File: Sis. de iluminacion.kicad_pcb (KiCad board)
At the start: 2 copper layers, 86.8 x 98.1 mm, 48 parts, among them J1 Screw_Terminal_01x02, J10 Screw_Terminal_01x02, J11 Screw_Terminal_01x02, J12 Screw_Terminal_01x02, J3 Screw_Terminal_01x02, J4 Conn_01x04, J5 Screw_Terminal_01x02, J7 Screw_Terminal_01x02, J8 Screw_Terminal_01x02, J9 Screw_Terminal_01x02, K10 Relay_DPDT, K11 Relay_DPDT, K8 Relay_DPDT, K9 Relay_DPDT, Q4 BC547, Q5 BC547, Q6 BC547, Q7 BC547, U1 ESP32_DEVKITC, U10 PC817, U11 PC817, U12 PC817, U13 PC817, U3 L7805

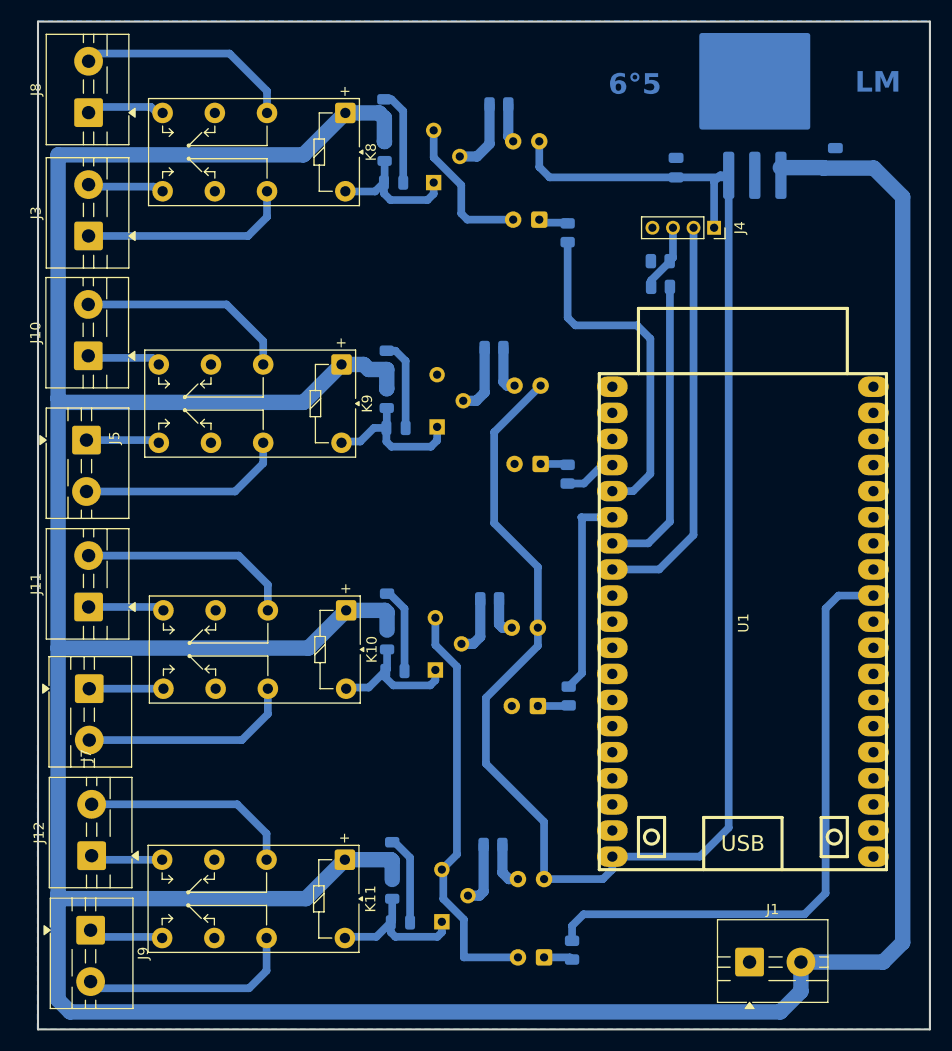
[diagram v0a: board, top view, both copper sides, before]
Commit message: Add files via upload
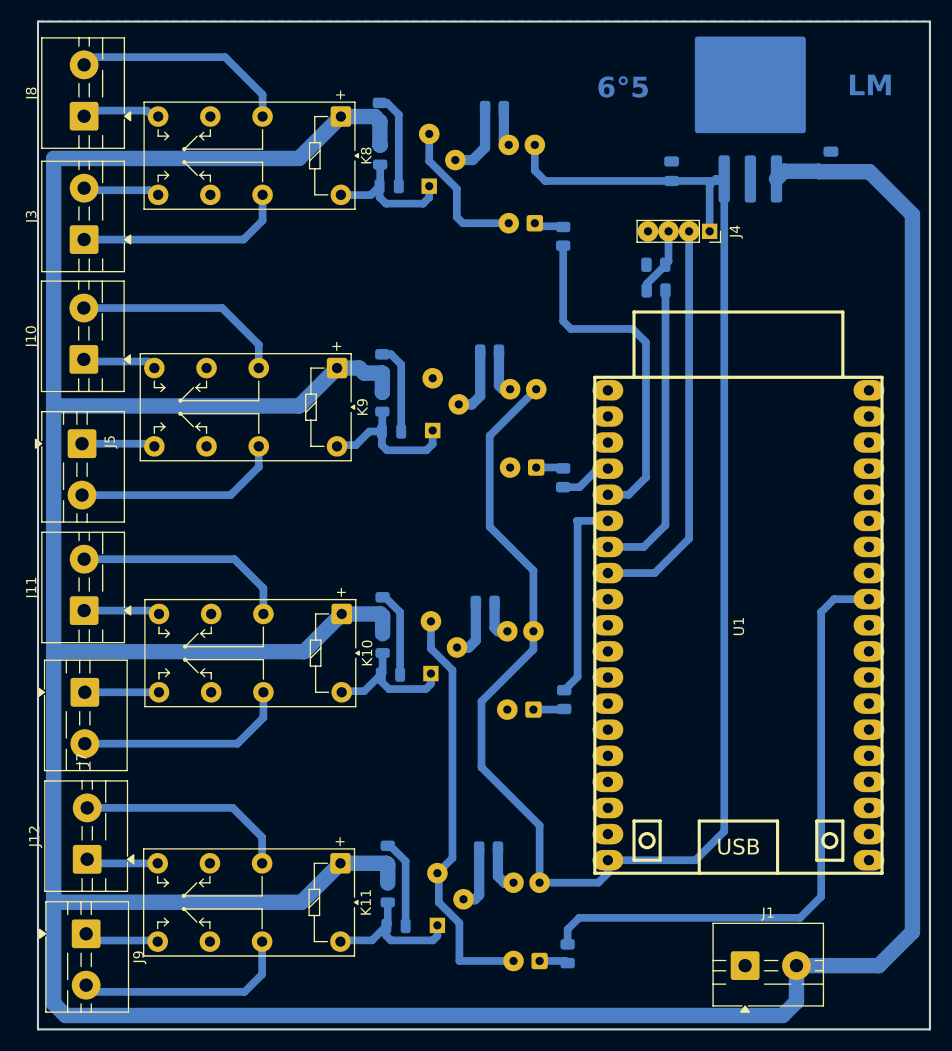
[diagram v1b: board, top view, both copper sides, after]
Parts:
- moved Q7 0.56 mm to (219.0, 129.6)
- moved D18 0.56 mm to (213.6, 78.7)
- moved D19 0.56 mm to (214.4, 105.2)
- moved D22 0.56 mm to (214.1, 126.4)
- moved J10 0.56 mm to (184.6, 74.5)
- moved J11 0.56 mm to (184.6, 99.0)
- moved J12 0.56 mm to (184.9, 123.2)
- moved J5 0.56 mm to (184.4, 82.7)
- moved J7 0.56 mm to (184.7, 106.9)
- moved K11 0.56 mm to (209.5, 123.5)
- moved K9 0.56 mm to (209.2, 75.4)
- moved R28 0.56 mm to (231.2, 86.0)
- moved R33 0.56 mm to (223.6, 98.2)
- moved C1 0.56 mm to (257.3, 55.2)
- moved D15 0.56 mm to (214.3, 57.7)
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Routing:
- net +12V: track 398.2 -> 400.0 mm
